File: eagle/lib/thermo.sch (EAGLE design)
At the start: 14 parts, among them U1 MLX90640ESF-BAB-000-TU

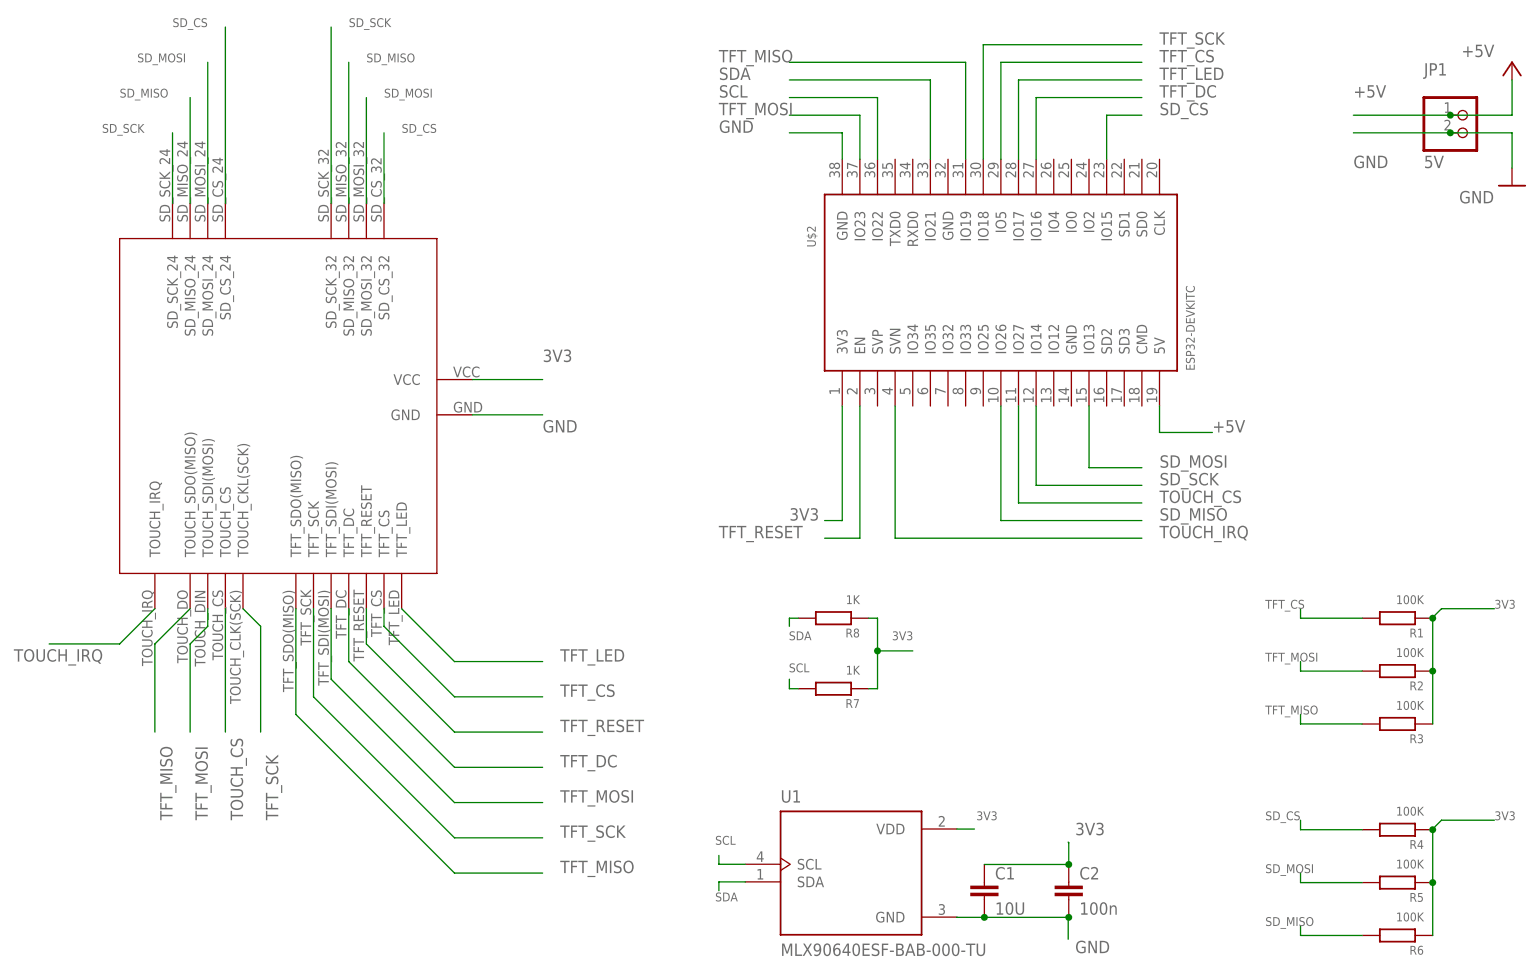
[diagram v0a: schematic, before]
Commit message: Updated scheme 0.0.2
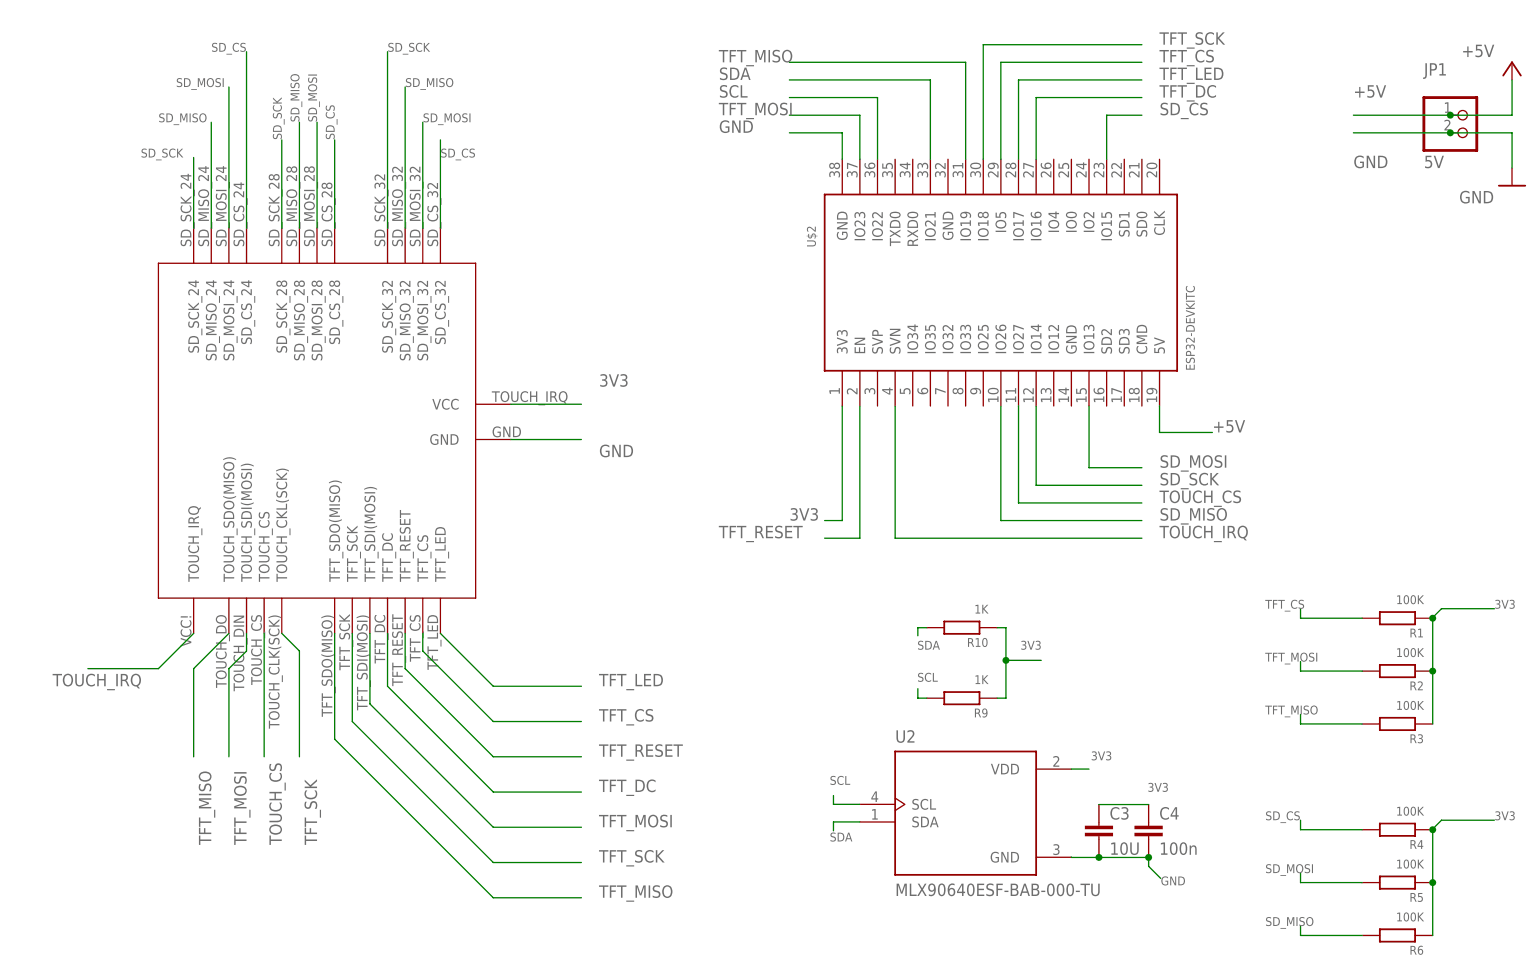
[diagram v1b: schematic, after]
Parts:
- removed C1: 10U, capacitor-wima:C2,5-3
- removed C2: 100n, capacitor-wima:C2,5-3
- removed R7, R8: 1K, rcl:R-EU_0204/7
- removed U1: MLX90640ESF-BAB-000-TU, teploblinEkran:MLX90640ESF-BAB-000-TU
- added C3: 10U, capacitor-wima:C2,5-3
- added C4: 100n, capacitor-wima:C2,5-3
- added R10, R9: 1K, rcl:R-EU_0204/7
- added U2: MLX90640ESF-BAB-000-TU, teploblinEkran:MLX90640ESF-BAB-000-TU
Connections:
- net 3V3: now also C3.1, C4.1, R10.1, R9.1, U2.VDD; no longer C1.1, C2.1, R7.1, R8.1, U1.VDD
- net GND: now also C3.2, C4.2, U2.GND; no longer C1.2, C2.2, U1.GND
- net SCL: now also R9.2, U2.SCL; no longer R7.2, U1.SCL
- net SDA: now also R10.2, U2.SDA; no longer R8.2, U1.SDA
- net SD_CS: now also U$1.SD_CS_28
- net SD_MISO: now also U$1.SD_MISO_28
- net SD_MOSI: now also U$1.SD_MOSI_28
- net SD_SCK: now also U$1.SD_SCK_28

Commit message: Fixed scheme 0.1.2
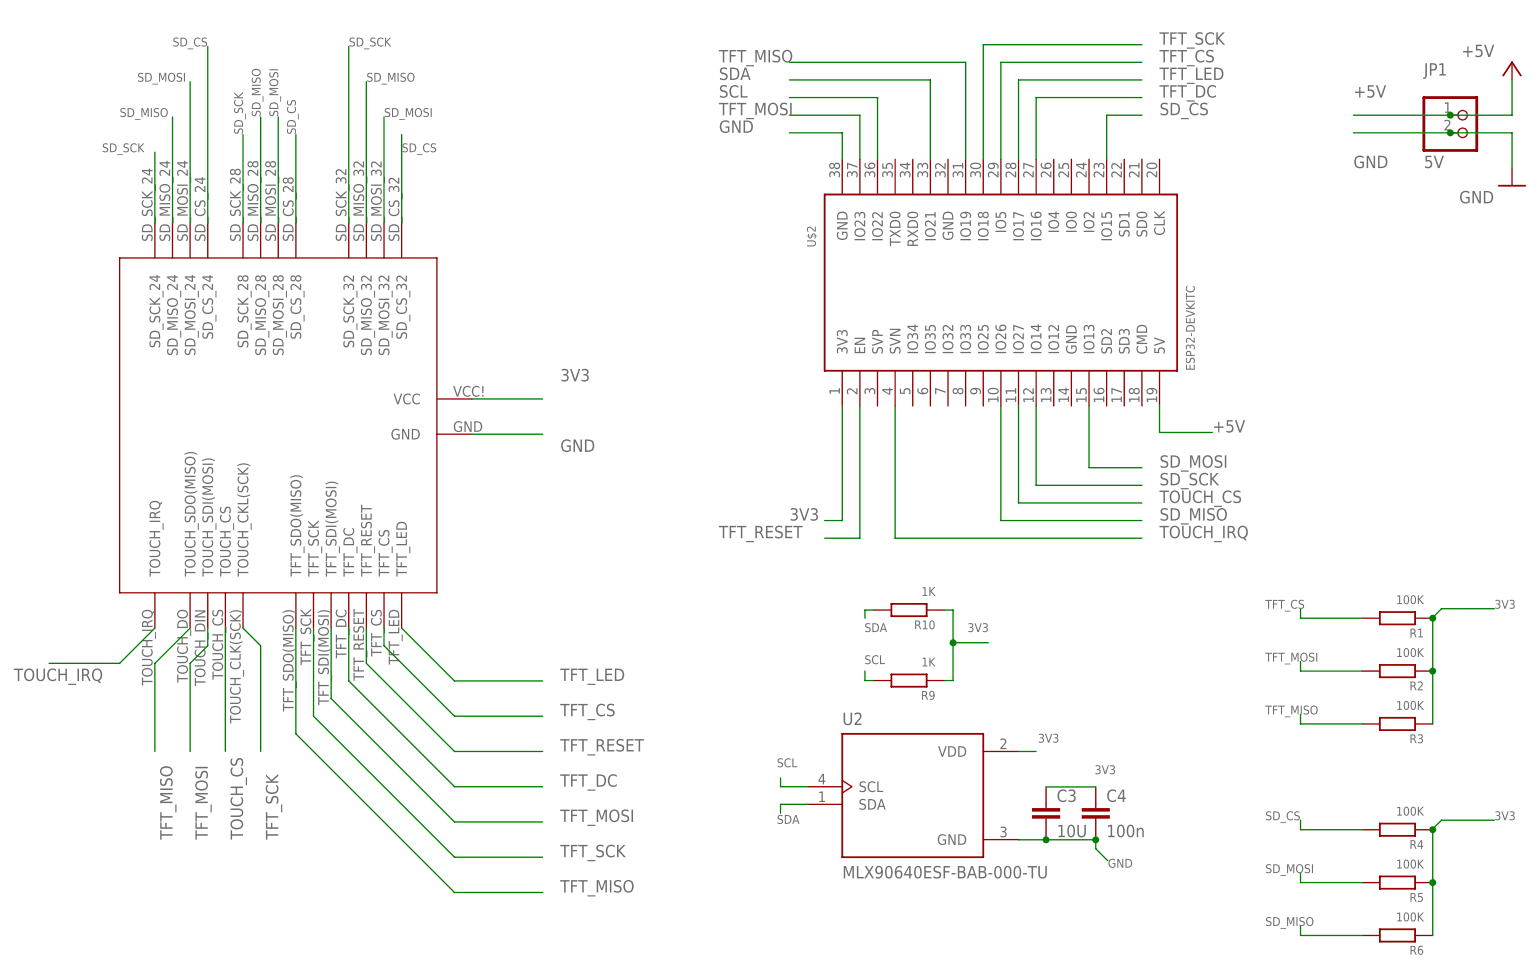
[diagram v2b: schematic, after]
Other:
- moved on the sheet: C3, C4, R10, R9, U2
